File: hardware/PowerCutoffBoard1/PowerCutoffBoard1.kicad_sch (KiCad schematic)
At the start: 47 parts, among them J1 Conn_Coaxial, J2 Conn_01x03, J3 Conn_01x04, J4 Conn_01x04, J5 Conn_01x04, J6 Conn_01x04, SW1 SW_Push, SW2 SW_Push, SW3 SW_DIP_x04, U1 STM32F303K8Tx, U2 Wio-E5, U3 3.3V, U4 MIC4427, U5 MCP2562-E-SN

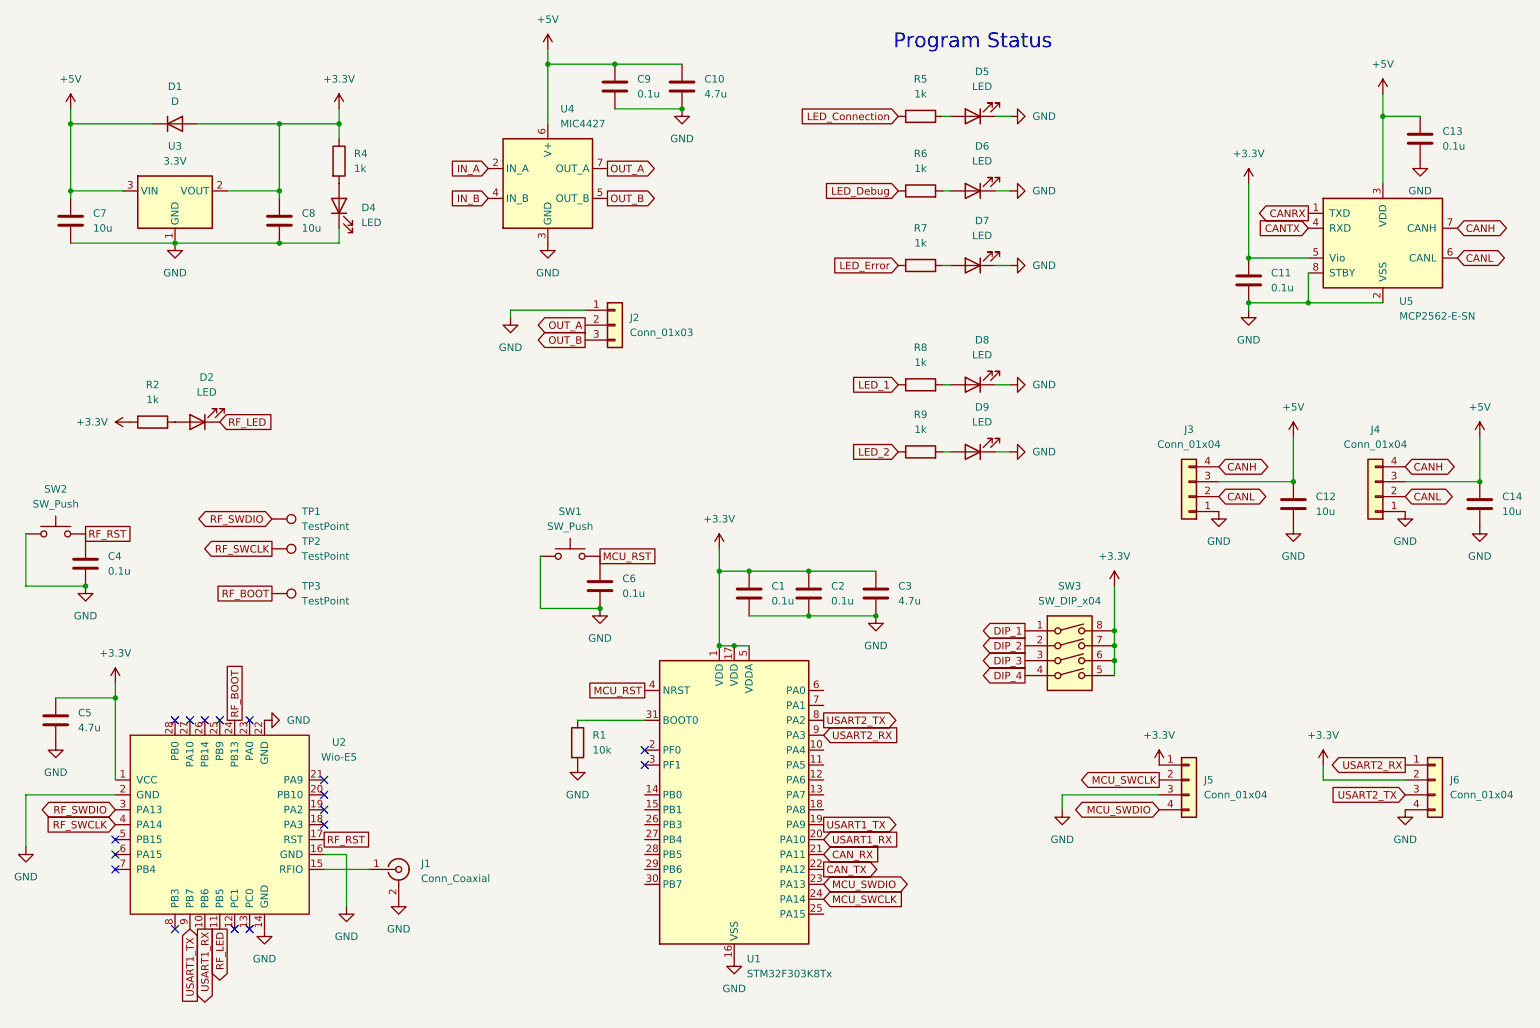
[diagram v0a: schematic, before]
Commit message: update
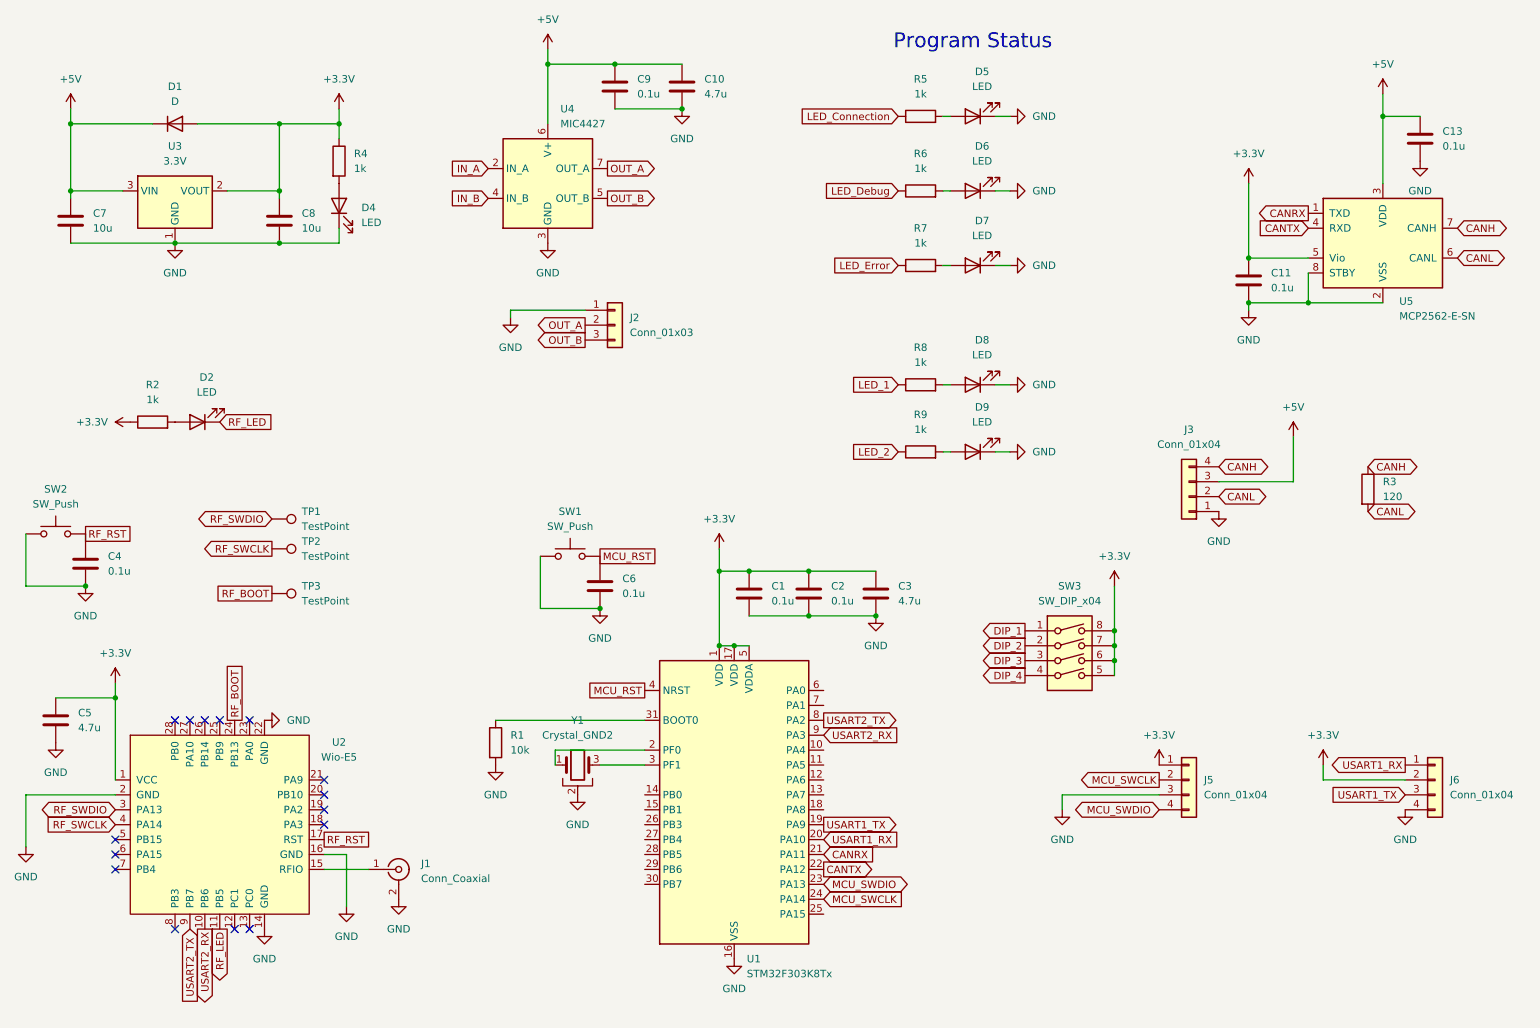
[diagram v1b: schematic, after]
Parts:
- removed C12, C14: 10u, Capacitor_SMD:C_0805_2012Metric_Pad1.18x1.45mm_HandSolder, symbol Device:C
- removed J4: Conn_01x04, Connector_JST:JST_XH_S4B-XH-A_1x04_P2.50mm_Horizontal, symbol Connector_Generic:Conn_01x04
- added R3: 120, Resistor_SMD:R_0603_1608Metric_Pad0.98x0.95mm_HandSolder, symbol Device:R
- added Y1: Crystal_GND2, Crystal:Resonator_SMD_Murata_CSTxExxV-3Pin_3.0x1.1mm_HandSoldering, symbol Device:Crystal_GND2
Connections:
- net CAN_RX is gone; now on net CANRX: U1.21 (PA11)
- net CAN_TX is gone; now on net CANTX: U1.22 (PA12)
- net CANH: now also R3.1
- net CANL: now also R3.2
- net GND: now also Y1.2
- net USART1_RX: now also J6.1 (Pin_1); no longer U2.10 (PB6)
- net USART1_TX: now also J6.3 (Pin_3); no longer U2.9 (PB7)
- net USART2_RX: now also U2.10 (PB6); no longer J6.1 (Pin_1)
- net USART2_TX: now also U2.9 (PB7); no longer J6.3 (Pin_3)
- net at U1.2 (PF0): now also Y1.1
- net at U1.3 (PF1): now also Y1.3
- no-connect marks 17 -> 15
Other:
- moved on the sheet: R1

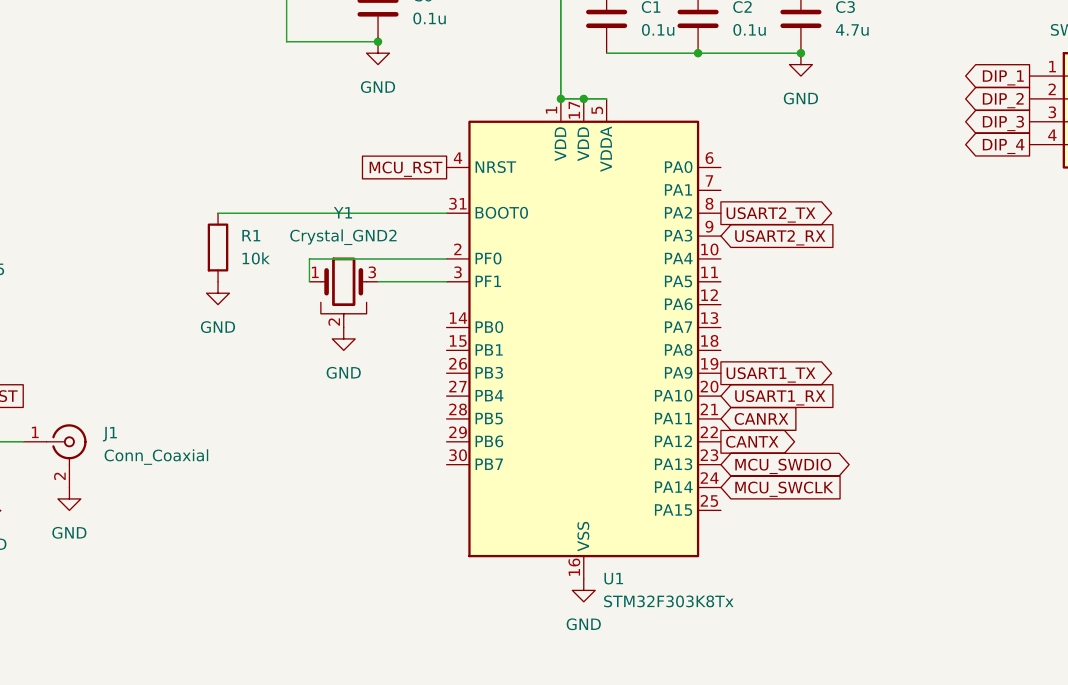
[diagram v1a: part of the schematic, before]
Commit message: fix:schematic
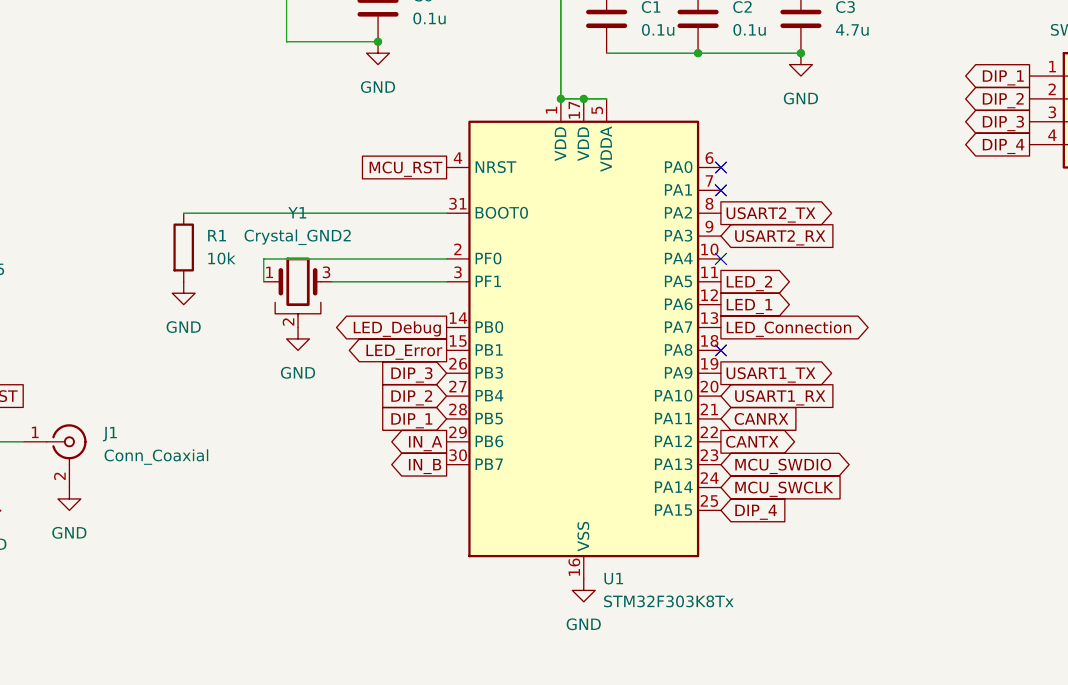
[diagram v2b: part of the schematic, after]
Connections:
- net DIP_1: now also U1.28 (PB5)
- net DIP_2: now also U1.27 (PB4)
- net DIP_3: now also U1.26 (PB3)
- net DIP_4: now also U1.25 (PA15)
- net IN_A: now also U1.29 (PB6)
- net IN_B: now also U1.30 (PB7)
- net LED_1: now also U1.12 (PA6)
- net LED_2: now also U1.11 (PA5)
- net LED_Connection: now also U1.13 (PA7)
- net LED_Debug: now also U1.14 (PB0)
- net LED_Error: now also U1.15 (PB1)
- no-connect marks 15 -> 19
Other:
- moved on the sheet: R1, Y1
